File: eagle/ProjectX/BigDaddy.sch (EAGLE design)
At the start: 4 parts, among them U1 TC4427AEOA

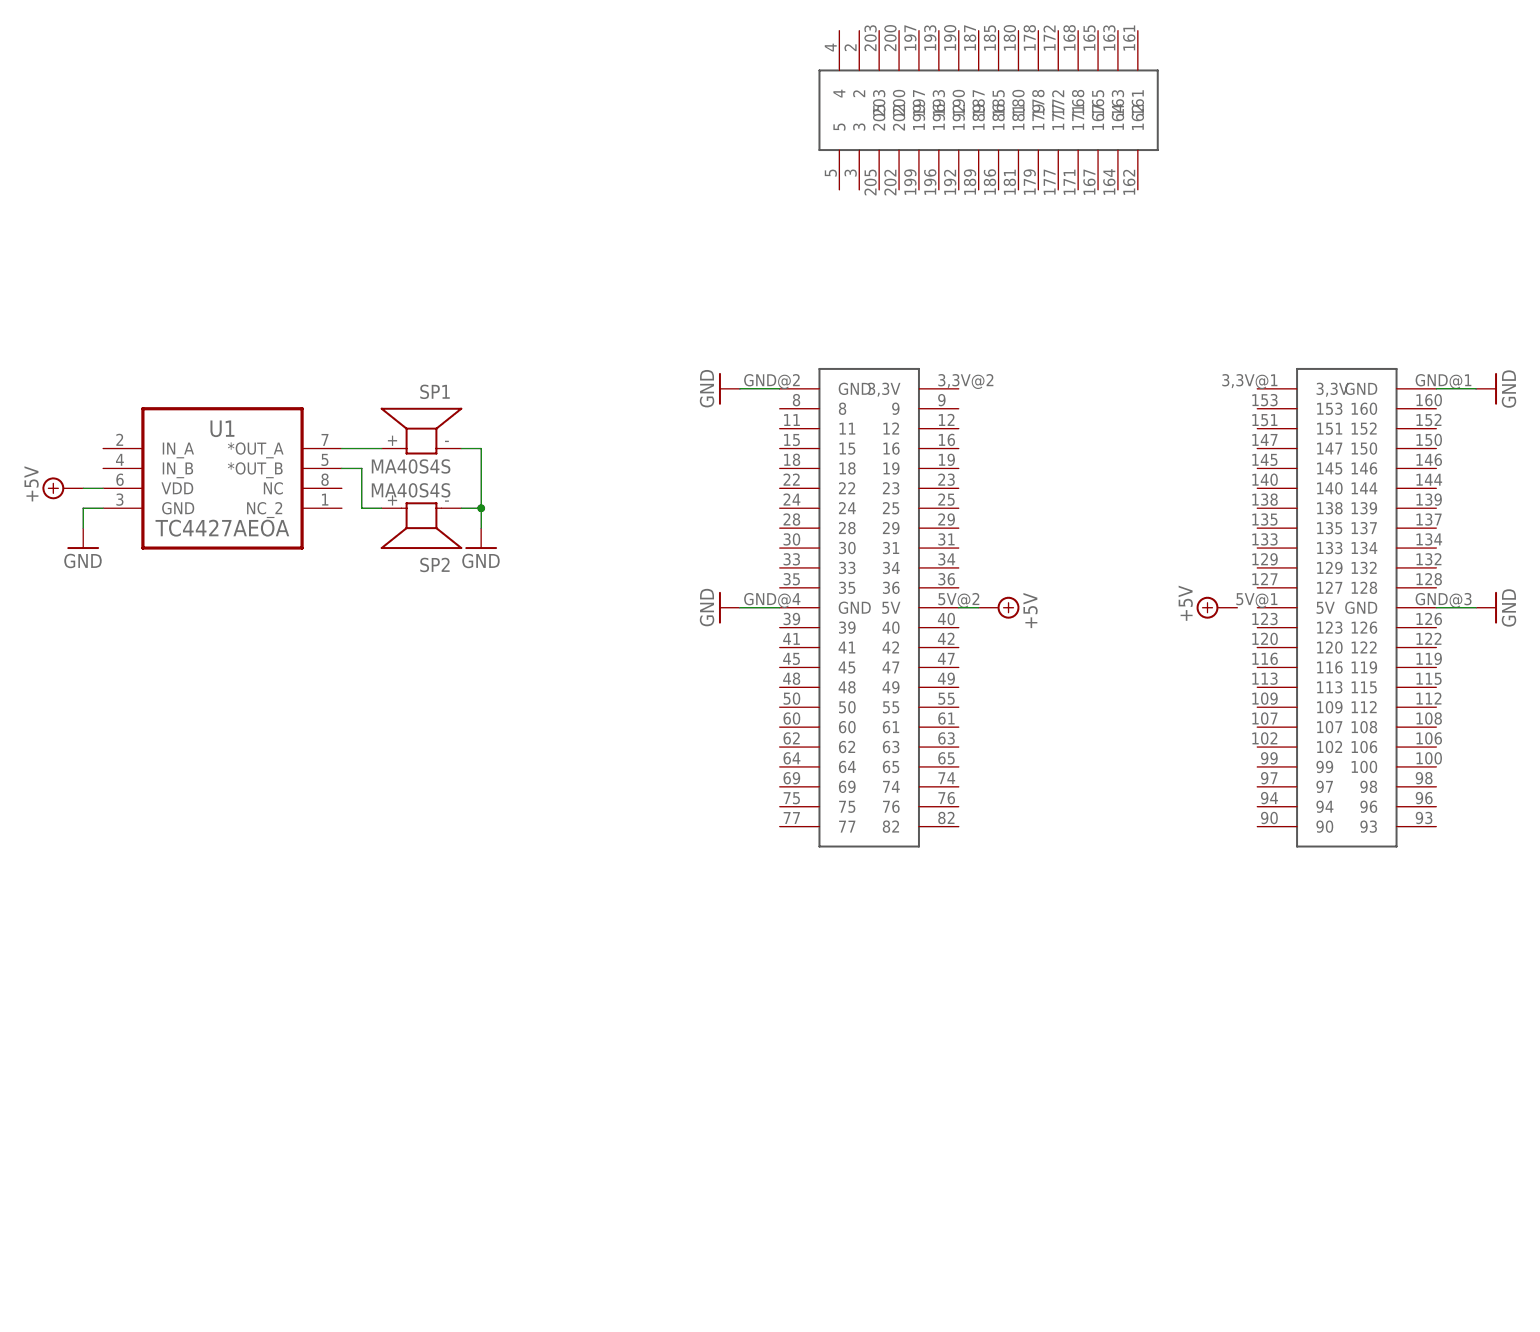
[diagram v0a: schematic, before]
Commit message: Working on the big board
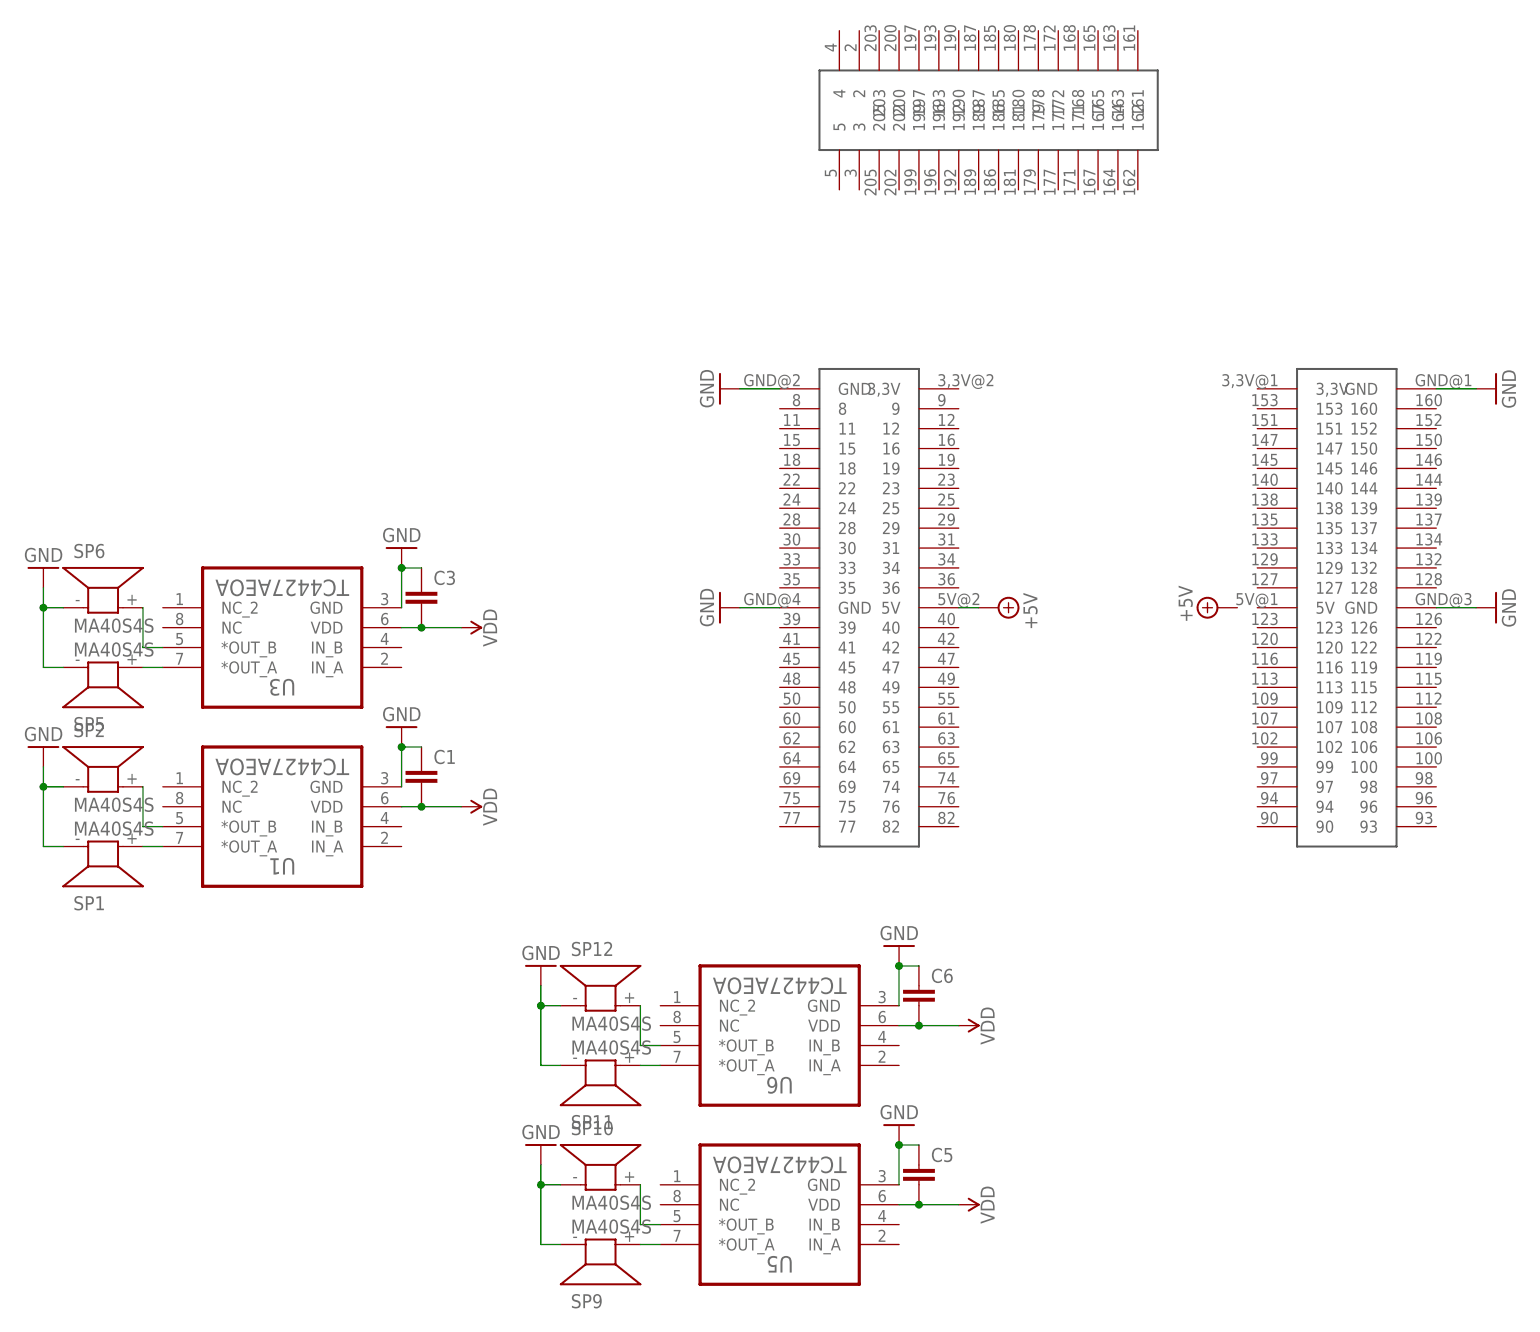
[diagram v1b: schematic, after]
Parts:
- added C1, C3, C5, C6: (no value), resistor:C-EUC0805
- added SP10, SP11, SP12, SP5, SP6, SP9: MA40S4S, Parts:MA40S4S
- added U3, U5, U6: TC4427AEOA, Parts:TC4427AEOA
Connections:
- new net N$10: SP6.2, U3.*OUT_B
- new net N$13: SP11.2, U6.*OUT_A
- new net N$14: SP12.2, U6.*OUT_B
- new net N$7: SP9.2, U5.*OUT_A
- new net N$8: SP10.2, U5.*OUT_B
- new net N$9: SP5.2, U3.*OUT_A
- new net VDD: C1.2, C3.2, C5.2, C6.2, U1.VDD, U3.VDD, U5.VDD, U6.VDD
- net +5V: no longer U1.VDD
- net GND: now also C1.1, C3.1, C5.1, C6.1, SP10.1, SP11.1, SP12.1, SP5.1, SP6.1, SP9.1, U3.GND, U5.GND, U6.GND
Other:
- moved on the sheet: SP1, SP2, U1
